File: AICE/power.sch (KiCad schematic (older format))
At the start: 22 parts

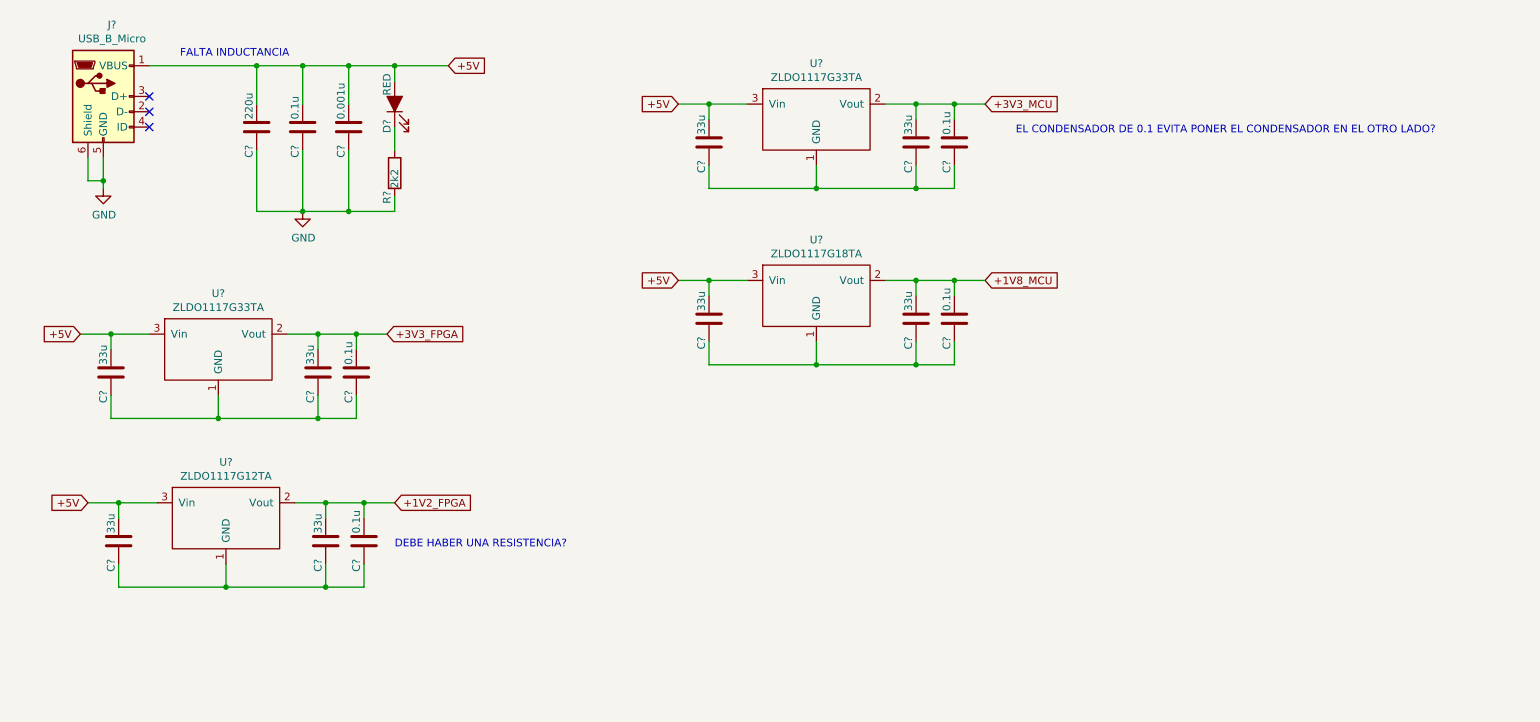
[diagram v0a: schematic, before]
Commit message: Add files via upload
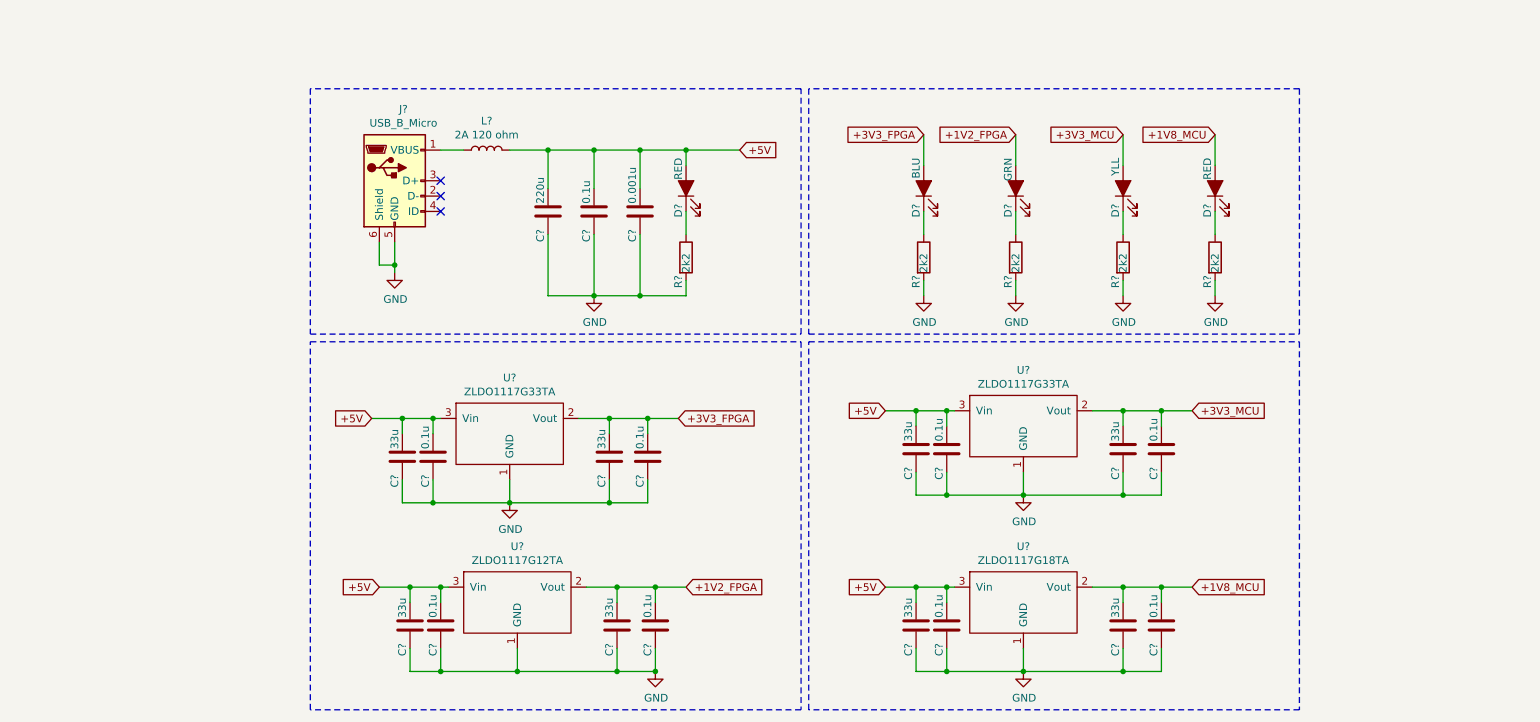
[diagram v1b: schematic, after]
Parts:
- added C? (x4): 0.1u, symbol Device:C
- added D?: BLU, symbol Device:LED_ALT
- added D?: GRN, symbol Device:LED_ALT
- added D?: YLL, symbol Device:LED_ALT
- added D?: RED, symbol Device:LED_ALT
- added L?: 2A 120 ohm, symbol Device:L
- added R? (x4): 2k2, symbol Device:R
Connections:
- net +1V2_FPGA: now also D?.2 (A)
- net +1V8_MCU: now also D?.2 (A)
- net +3V3_FPGA: now also D?.2 (A)
- net +3V3_MCU: now also D?.2 (A)
- net +5V: now also C?.1, C?.1, C?.1, C?.1, L?.2; no longer J?.1 (VBUS)
- net GND: now also C?.2, C?.2, C?.2, C?.2, C?.2, C?.2, C?.2, C?.2, C?.2, C?.2, C?.2, C?.2, U?.1 (GND), U?.1 (GND), U?.1 (GND), U?.1 (GND), C?.2, C?.2, C?.2, C?.2, R?.2, R?.2, R?.2, R?.2
- new net: J?.1 (VBUS), L?.1
- new net: D?.1 (K), R?.1 (x4)
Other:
- note removed: "DEBE HABER UNA RESISTENCIA?"
- note removed: "EL CONDENSADOR DE 0.1 EVITA PONER EL CONDENSADOR EN EL OTRO LADO?"
- note removed: "FALTA INDUCTANCIA"
- moved on the sheet: C?, D?, J?, R?, U?

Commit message: Add files via upload
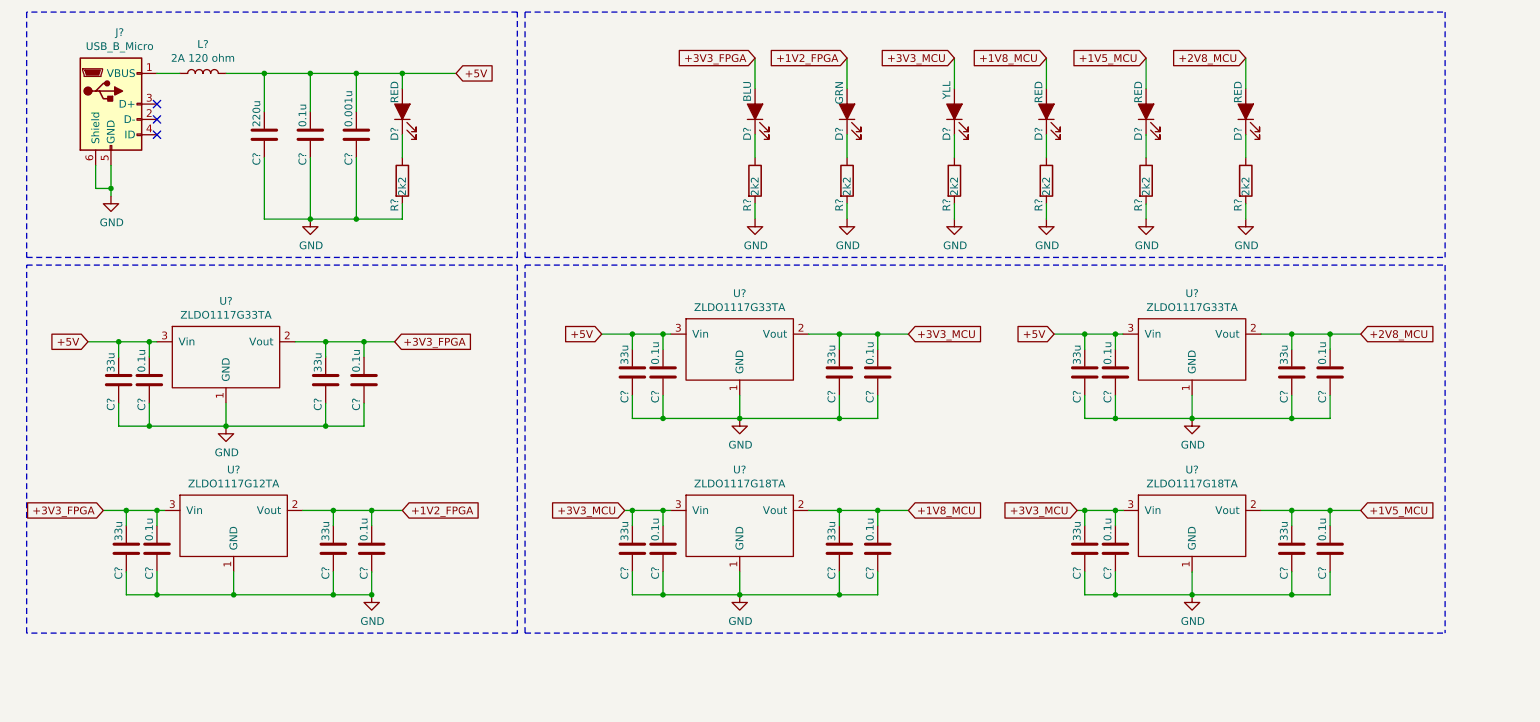
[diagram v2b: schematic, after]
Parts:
- added C? (x4): 33u, symbol Device:C
- added C? (x4): 0.1u, symbol Device:C
- added D? (x2): RED, symbol Device:LED_ALT
- added R? (x2): 2k2, symbol Device:R
- added U?: ZLDO1117G18TA, symbol LDO:ZLDO1117G18TA
- added U?: ZLDO1117G33TA, symbol LDO:ZLDO1117G33TA
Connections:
- net +3V3_FPGA: now also C?.1, C?.1, U?.3 (Vin)
- net +3V3_MCU: now also C?.1, C?.1, U?.3 (Vin), C?.1, C?.1, U?.3 (Vin)
- net +5V: now also C?.1, C?.1, U?.3 (Vin); no longer C?.1, C?.1, C?.1, C?.1, U?.3 (Vin), U?.3 (Vin)
- net GND: now also C?.2, C?.2, C?.2, C?.2, C?.2, C?.2, C?.2, C?.2, R?.2, R?.2, U?.1 (GND), U?.1 (GND)
- new net: D?.1 (K), R?.1 (x2)
- new net +1V5_MCU: C?.1, C?.1, D?.2 (A), U?.2 (Vout)
- new net +2V8_MCU: C?.1, C?.1, D?.2 (A), U?.2 (Vout)
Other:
- moved on the sheet: C?, D?, J?, L?, R?, U?

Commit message: Add files via upload
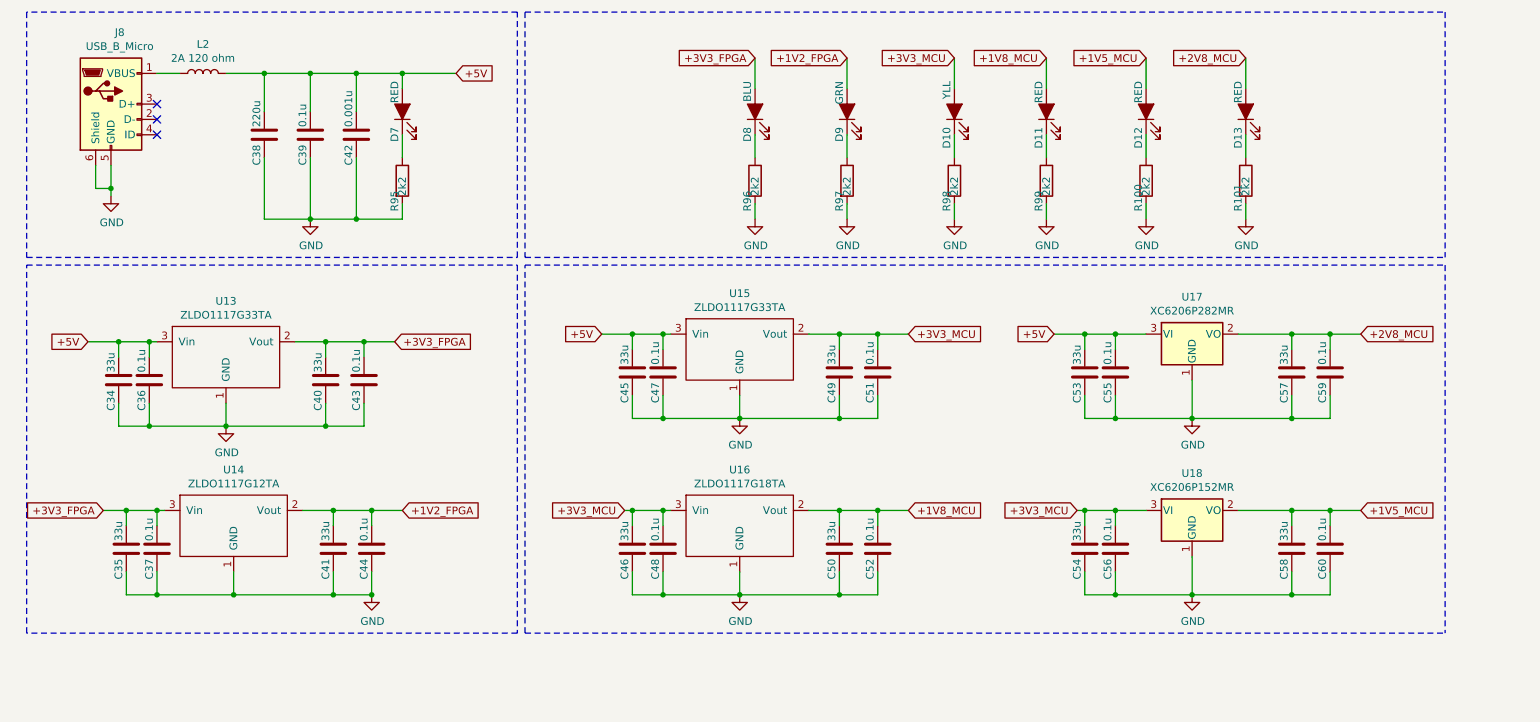
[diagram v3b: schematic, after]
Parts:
- removed U? (x3): ZLDO1117G33TA, symbol LDO:ZLDO1117G33TA
- removed U? (x2): ZLDO1117G18TA, symbol LDO:ZLDO1117G18TA
- removed U?: ZLDO1117G12TA, symbol LDO:ZLDO1117G12TA
- added U13, U15: ZLDO1117G33TA, Package_TO_SOT_SMD:SOT-223, symbol LDO:ZLDO1117G33TA
- added U14: ZLDO1117G12TA, Package_TO_SOT_SMD:SOT-223, symbol LDO:ZLDO1117G12TA
- added U16: ZLDO1117G18TA, Package_TO_SOT_SMD:SOT-223, symbol LDO:ZLDO1117G18TA
- added U17: XC6206P282MR, Package_TO_SOT_SMD:SOT-23, symbol Regulator_Linear:XC6206PxxxMR
- added U18: XC6206P152MR, Package_TO_SOT_SMD:SOT-23, symbol Regulator_Linear:XC6206PxxxMR
- J8: renamed from J?; footprint (none) -> Connector_USB:USB_Micro-B_Molex_47346-0001
- gave numbers to parts that had none: 42
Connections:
- net +1V2_FPGA: now also U14.2 (Vout)
- net +1V5_MCU: now also U18.2 (VO)
- net +1V8_MCU: now also U16.2 (Vout)
- net +2V8_MCU: now also U17.2 (VO)
- net +3V3_FPGA: now also U13.2 (Vout), U14.3 (Vin)
- net +3V3_MCU: now also U15.2 (Vout), U16.3 (Vin), U18.3 (VI)
- net +5V: now also U13.3 (Vin), U15.3 (Vin), U17.3 (VI)
- net GND: now also U13.1 (GND), U14.1 (GND), U15.1 (GND), U16.1 (GND), U17.1 (GND), U18.1 (GND)

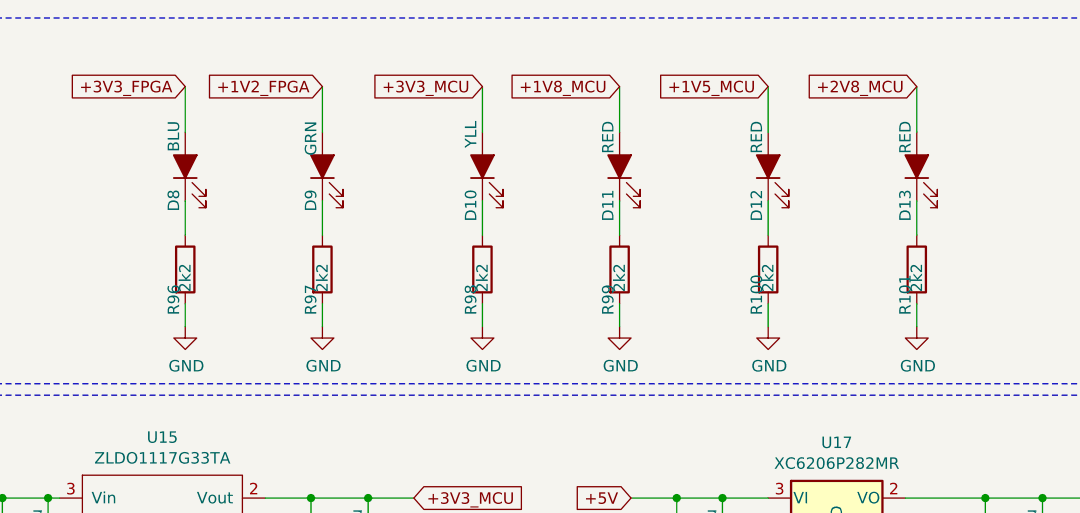
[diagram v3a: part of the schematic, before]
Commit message: Add files via upload
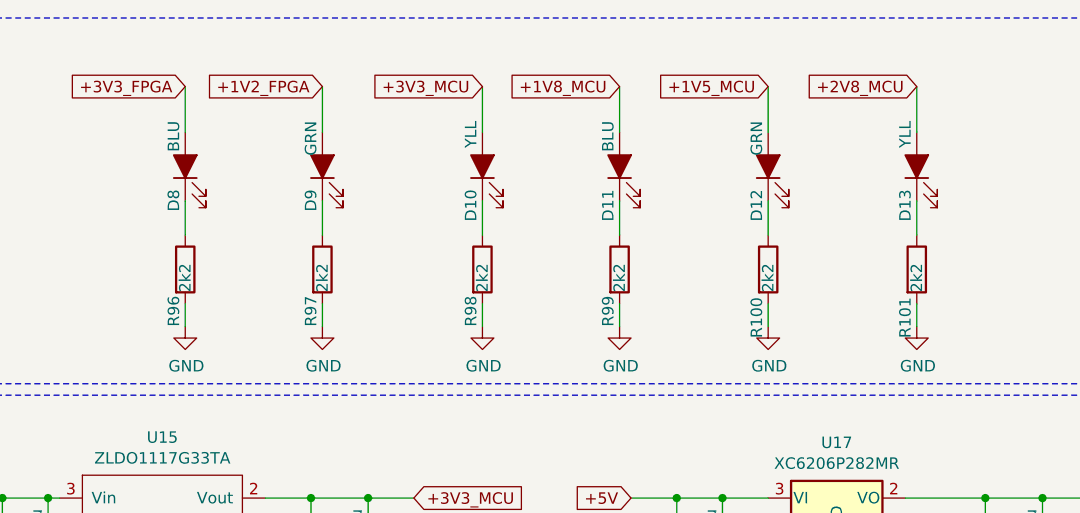
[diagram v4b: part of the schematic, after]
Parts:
- C34, C35, C36, C37, C39, C40, C41, C43, C44, C45, C46, C47, C48, C49, C50, C51, C52, C53, C54, C55, C56, C57, C58, C59, C60: footprint (none) -> Capacitor_SMD:C_0805_2012Metric_Pad1.15x1.40mm_HandSolder
- C38: footprint (none) -> Capacitor_SMD:C_1206_3216Metric_Pad1.42x1.75mm_HandSolder
- C42: footprint (none) -> Capacitor_SMD:C_0603_1608Metric_Pad1.05x0.95mm_HandSolder
- D10, D7, D8, D9: footprint (none) -> LED_SMD:LED_0603_1608Metric_Pad1.05x0.95mm_HandSolder
- D11: value RED -> BLU; footprint (none) -> LED_SMD:LED_0603_1608Metric_Pad1.05x0.95mm_HandSolder
- D12: value RED -> GRN; footprint (none) -> LED_SMD:LED_0603_1608Metric_Pad1.05x0.95mm_HandSolder
- D13: value RED -> YLL; footprint (none) -> LED_SMD:LED_0603_1608Metric_Pad1.05x0.95mm_HandSolder
- R100, R101, R95, R96, R97, R98, R99: footprint (none) -> Resistor_SMD:R_0805_2012Metric_Pad1.15x1.40mm_HandSolder

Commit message: Add files via upload
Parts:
- L2: footprint (none) -> Inductor_SMD:L_0805_2012Metric_Pad1.15x1.40mm_HandSolder
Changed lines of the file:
@@
 F 0 "L2" V 2140 1100 50  0000 C CNN
 F 1 "2A 120 ohm" V 2049 1100 50  0000 C CNN
-F 2 "" H 1950 1100 50  0001 C CNN
+F 2 "Inductor_SMD:L_0805_2012Metric_Pad1.15x1.40mm_HandSolder" H 1950 1100 50  0001 C CNN
 F 3 "~" H 1950 1100 50  0001 C CNN
 	1    1950 1100
